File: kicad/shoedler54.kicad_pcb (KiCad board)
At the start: 2 copper layers, 139.1 x 121.9 mm, 63 parts

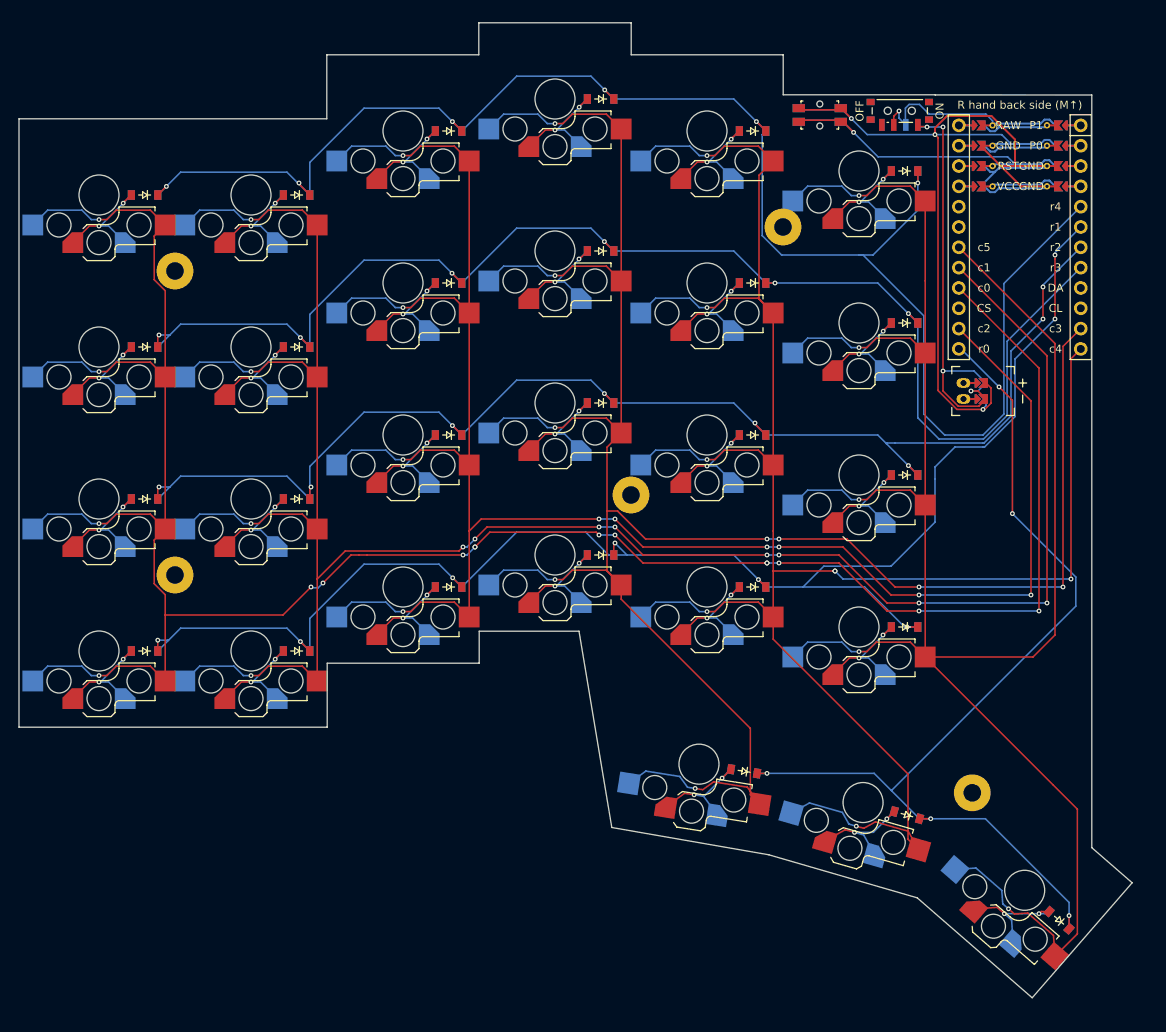
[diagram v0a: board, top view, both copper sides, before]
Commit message: v1
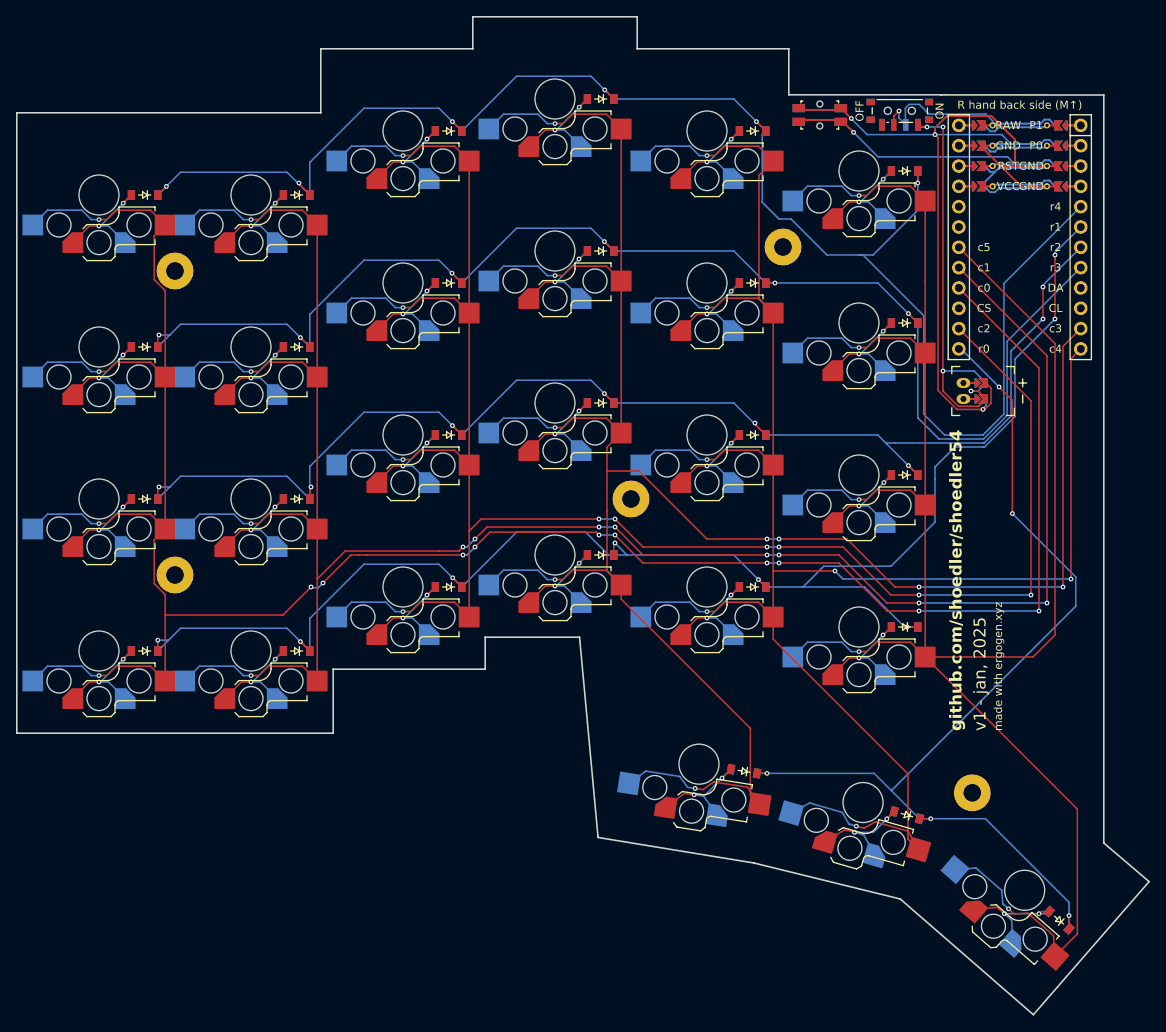
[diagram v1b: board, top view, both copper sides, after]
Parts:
- moved MH2 2.50 mm to (235.5, 99.5)
- moved MH5 0.50 mm to (216.5, 131.0)
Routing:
- net r4: track 208.3 -> 205.8 mm
- net c3: track 282.5 -> 284.6 mm
- net c4: vias 8 -> 7
- net c0: vias 16 -> 14
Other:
- board size 139.1 x 121.9 mm -> 141.5 x 124.7 mm
- board text added: "github.com/shoedler/shoedler54"
- board text added: "made with ergogen.xyz"
- board text added: "v1 - jan, 2025"
